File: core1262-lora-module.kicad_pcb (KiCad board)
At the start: 2 copper layers, 9 parts, among them J1 PWR, J2 SPI, J3 MISC_IO, U1 Core1262

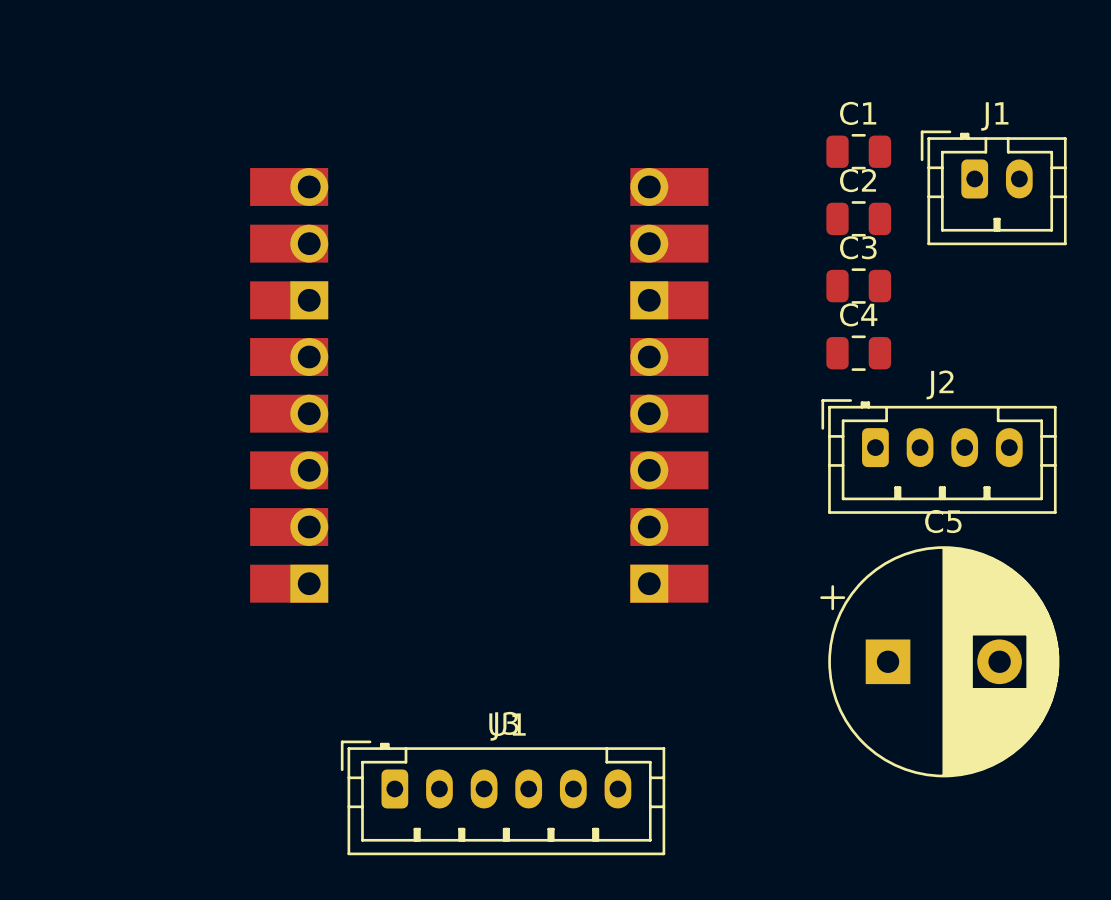
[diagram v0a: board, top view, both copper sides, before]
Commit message: PCB layout
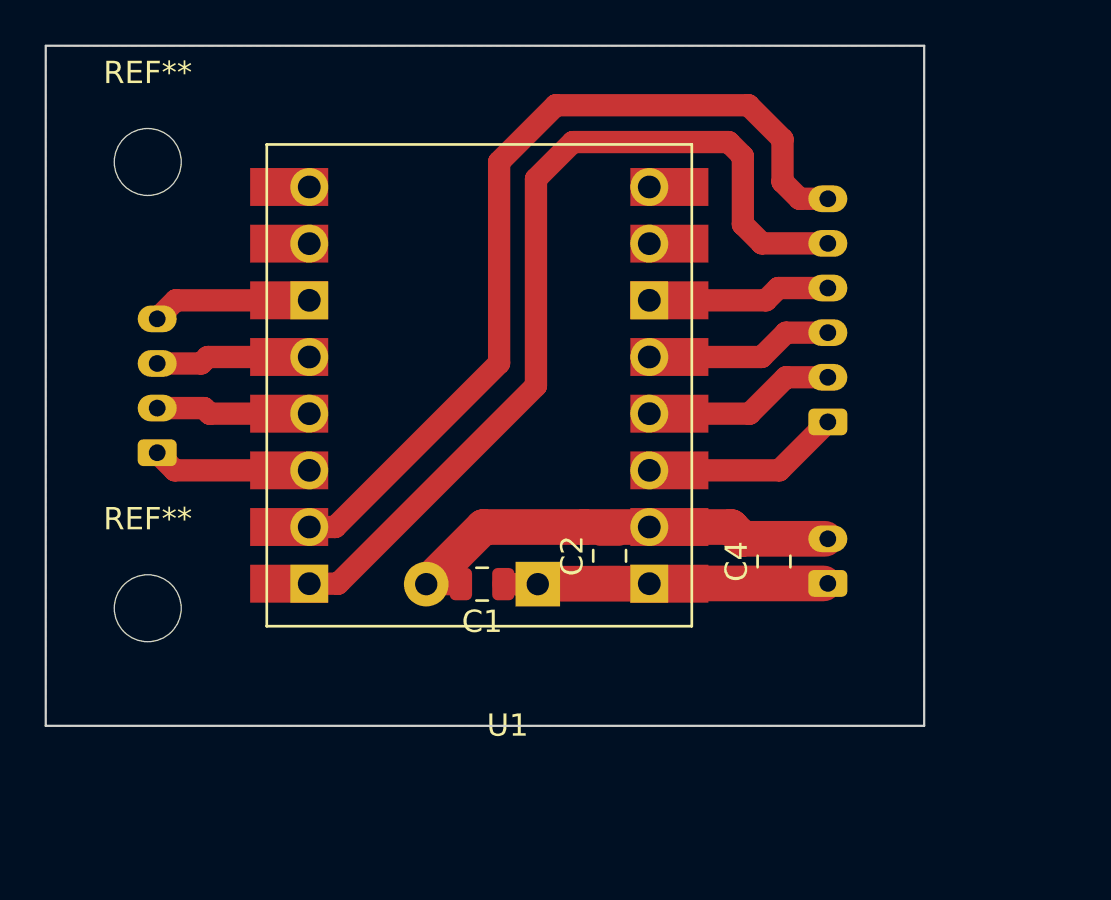
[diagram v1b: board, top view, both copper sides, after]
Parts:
- removed C3: 10uF, Capacitor_SMD:C_0805_2012Metric
- added REF**: MountingHole_3mm, MountingHole:MountingHole_3mm, F.Cu at (74.4, 59.5)
- added REF**: MountingHole_3mm, MountingHole:MountingHole_3mm, F.Cu at (74.4, 39.5)
- C5, J1, J2, J3: moved to B.Cu
- moved J2 32.2 mm to (74.8, 52.5), turned to 90 degrees
- moved C1 25.7 mm to (89.4, 58.4), turned to 180 degrees
- moved J3 25.4 mm to (104.9, 51.1), turned to 90 degrees
- moved J1 19.3 mm to (104.9, 58.4), turned to 90 degrees
- moved C2 18.8 mm to (95.1, 57.1), turned to 90 degrees
- moved C5 16.1 mm to (91.9, 58.4), turned to 180 degrees
- moved C4 10.1 mm to (102.5, 57.4), turned to 90 degrees
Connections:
- J1 pad 1: GND -> +3.3V
- J1 pad 2: +3.3V -> GND
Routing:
- net Net-(J3-Pin_5): track 0.00 -> 40.5 mm
- net Net-(J3-Pin_6): track 0.00 -> 39.2 mm
- net GND: track 0.00 -> 20.7 mm
- net +3.3V: track 0.00 -> 14.4 mm
- net DIO1: track 0.00 -> 8.90 mm
- net DIO2: track 0.00 -> 8.68 mm
- net TXen: track 0.00 -> 8.45 mm
- net RXen: track 0.00 -> 8.23 mm
- net Net-(J2-Pin_4): track 0.00 -> 7.16 mm
- net Net-(J2-Pin_1): track 0.00 -> 7.14 mm
- net Net-(J2-Pin_3): track 0.00 -> 6.94 mm
- net Net-(J2-Pin_2): track 0.00 -> 6.92 mm
- added copper zone on F.Cu, net GND
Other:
- board outline added: 39.4 x 30.5 mm
